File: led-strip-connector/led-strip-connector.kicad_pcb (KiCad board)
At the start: 2 copper layers, 39 x 49 mm, 4 parts, among them J1 Conn_01x03_Pin, J2 Conn_01x03_Pin, U1 NodeMCU_1.0_(ESP-12E)

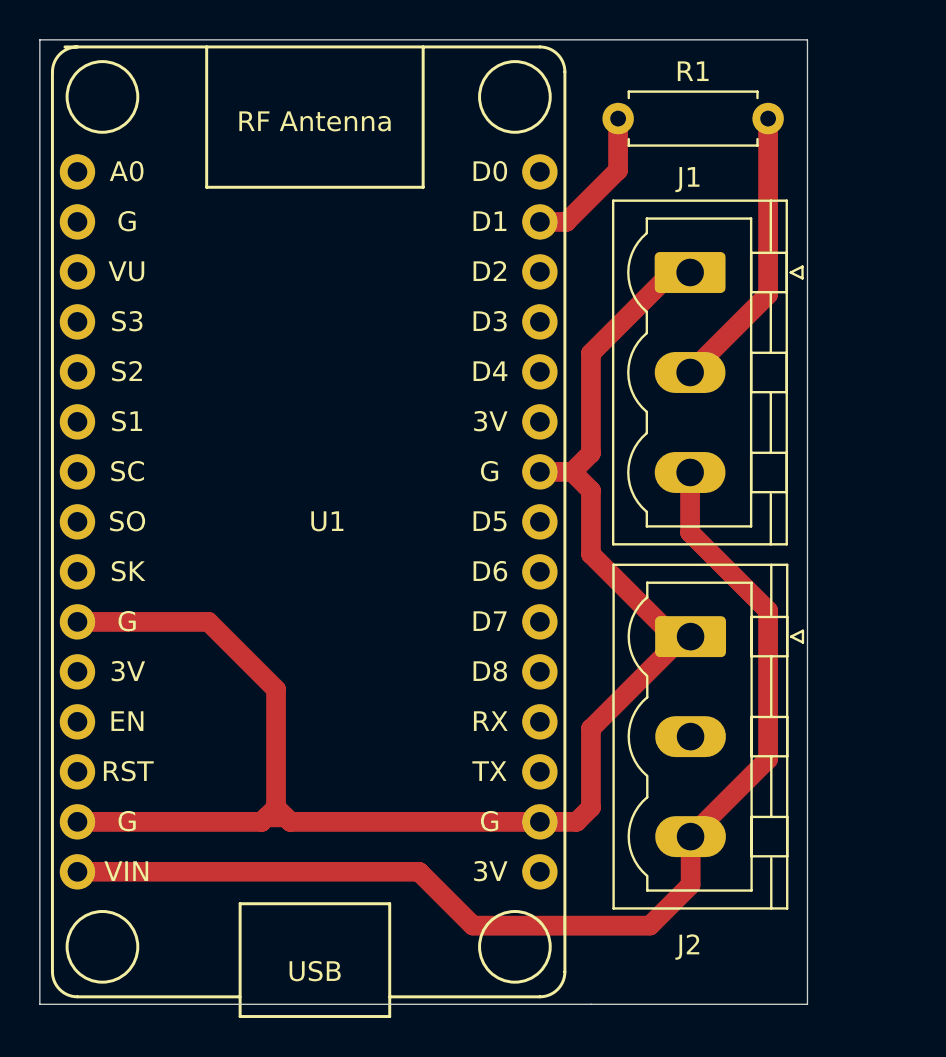
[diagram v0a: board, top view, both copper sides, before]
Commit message: new pcb
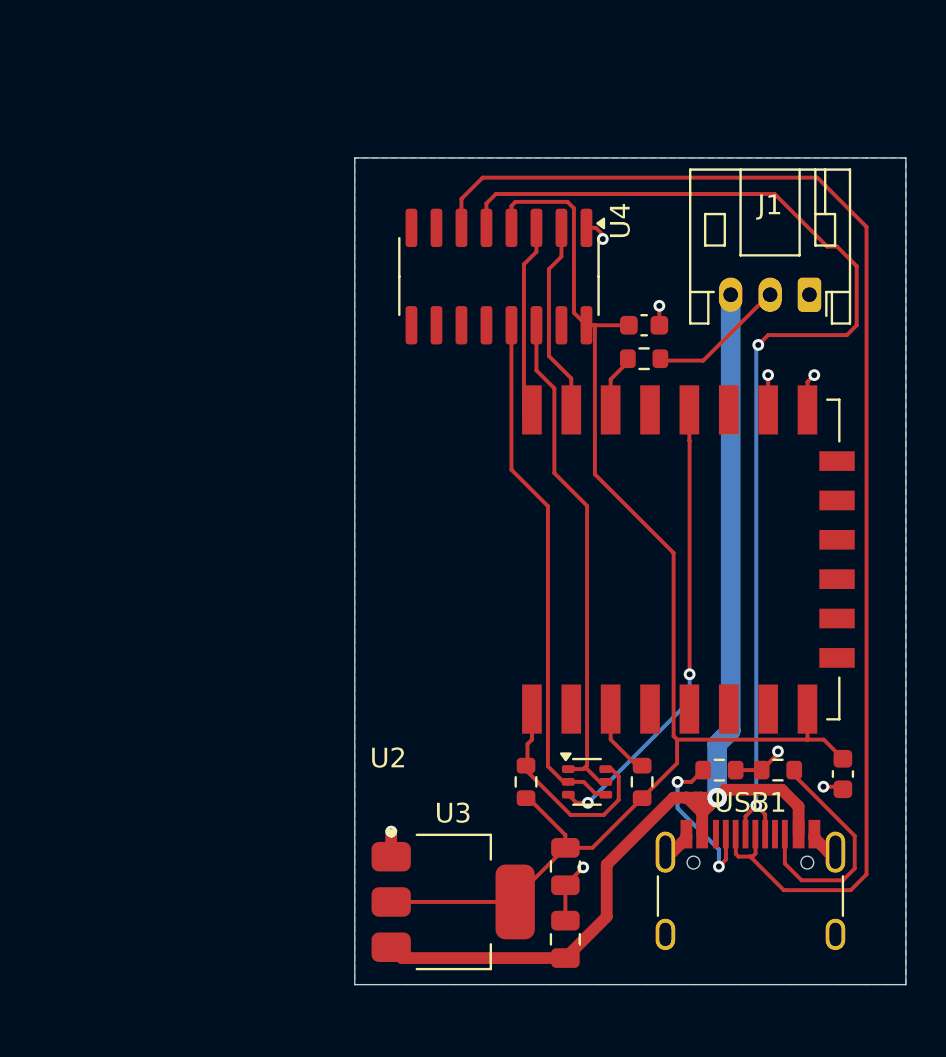
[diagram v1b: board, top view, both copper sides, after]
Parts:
- removed J2: Conn_01x03_Pin, Connector_Phoenix_MSTB:PhoenixContact_MSTBVA_2,5_3-G-5,08_1x03_P5.08mm_Vertical
- removed U1: NodeMCU_1.0_(ESP-12E), ESP8266:ESP12F-Devkit-V3
- added C1: 100n, Capacitor_SMD:C_0603_1608Metric, F.Cu at (158.7, 87.5)
- added C2: 100n, Capacitor_SMD:C_0603_1608Metric, F.Cu at (168.8, 110.3)
- added C3: 2.2u, Capacitor_SMD:C_0805_2012Metric, F.Cu at (154.7, 118.7)
- added C4: 2.2u, Capacitor_SMD:C_0805_2012Metric, F.Cu at (154.7, 115.0)
- added Q1: UMH3N, Package_TO_SOT_SMD:SOT-363_SC-70-6, F.Cu at (155.8, 110.7)
- added R2: 10K, Resistor_SMD:R_0603_1608Metric, F.Cu at (158.6, 110.7)
- added R3: 10K, Resistor_SMD:R_0603_1608Metric, F.Cu at (152.7, 110.7)
- added R4: 5K1, Resistor_SMD:R_0603_1608Metric, F.Cu at (165.5, 110.1)
- added R5: 5K1, Resistor_SMD:R_0603_1608Metric, F.Cu at (162.5, 110.1)
- added U2: ESP-12F, RF_Module:ESP-12E, F.Cu at (156.5, 99.4)
- added U3: LM1117MP-3.3, Package_TO_SOT_SMD:SOT-223-3_TabPin2, F.Cu at (149.0, 116.8)
- added U4: CH340C, Package_SO:SOIC-16_3.9x9.9mm_P1.27mm, F.Cu at (151.3, 85.0)
- added USB1: USB4105-GF-A, Connector_USB:USB_C_Receptacle_HRO_TYPE-C-31-M-12, F.Cu at (164.1, 117.4)
- J1: footprint Connector_Phoenix_MSTB:PhoenixContact_MSTBVA_2,5_3-G-5,08_1x03_P5.08mm_Vertical -> Connector_JST:JST_PH_S3B-PH-K_1x03_P2.00mm_Horizontal
- R1: footprint Resistor_THT:R_Axial_DIN0207_L6.3mm_D2.5mm_P7.62mm_Horizontal -> Resistor_SMD:R_0603_1608Metric
- moved R1 12.3 mm to (158.7, 89.2)
- moved J1 6.17 mm to (167.1, 86.0), turned to 180 degrees
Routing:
- net +3V3: track 0.00 -> 68.2 mm
- net GND: track 83.3 -> 17.0 mm, vias 0 -> 8
- net USBD-: track 0.00 -> 66.0 mm
- net USBD+: track 0.00 -> 56.9 mm, vias 0 -> 2
- net DTR: track 0.00 -> 26.7 mm
- net RTS: track 0.00 -> 25.8 mm
- net Net-(Q1B-C2): track 0.00 -> 23.3 mm, vias 0 -> 2
- net Net-(USB1-CC2): track 0.00 -> 11.9 mm
- net TX: track 0.00 -> 11.2 mm
- net Net-(Q1A-C1): track 0.00 -> 11.2 mm
- net RX: track 0.00 -> 9.98 mm
- net Net-(USB1-CC1): track 0.00 -> 8.25 mm, vias 0 -> 2
- net Net-(J1-Pin_2): track 14.5 -> 7.00 mm
- net Net-(U2-GPIO5): track 7.68 -> 2.96 mm
- net Net-(U2-EN): track 0.00 -> 3.70 mm
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- added copper zone on B.Cu, net GND
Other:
- board size 39 x 49 mm -> 28 x 42 mm
